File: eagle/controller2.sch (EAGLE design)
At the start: 27 parts, among them K1 SRD-05VDC-SL-C, K2 SRD-05VDC-SL-C, K3 SRD-05VDC-SL-C, K4 SRD-05VDC-SL-C, T1 BC547, T2 BC547, T3 BC547, T4 BC547, X1 VCC, X2 IN1, X3 IN2, X4 IN3, X5 IN4

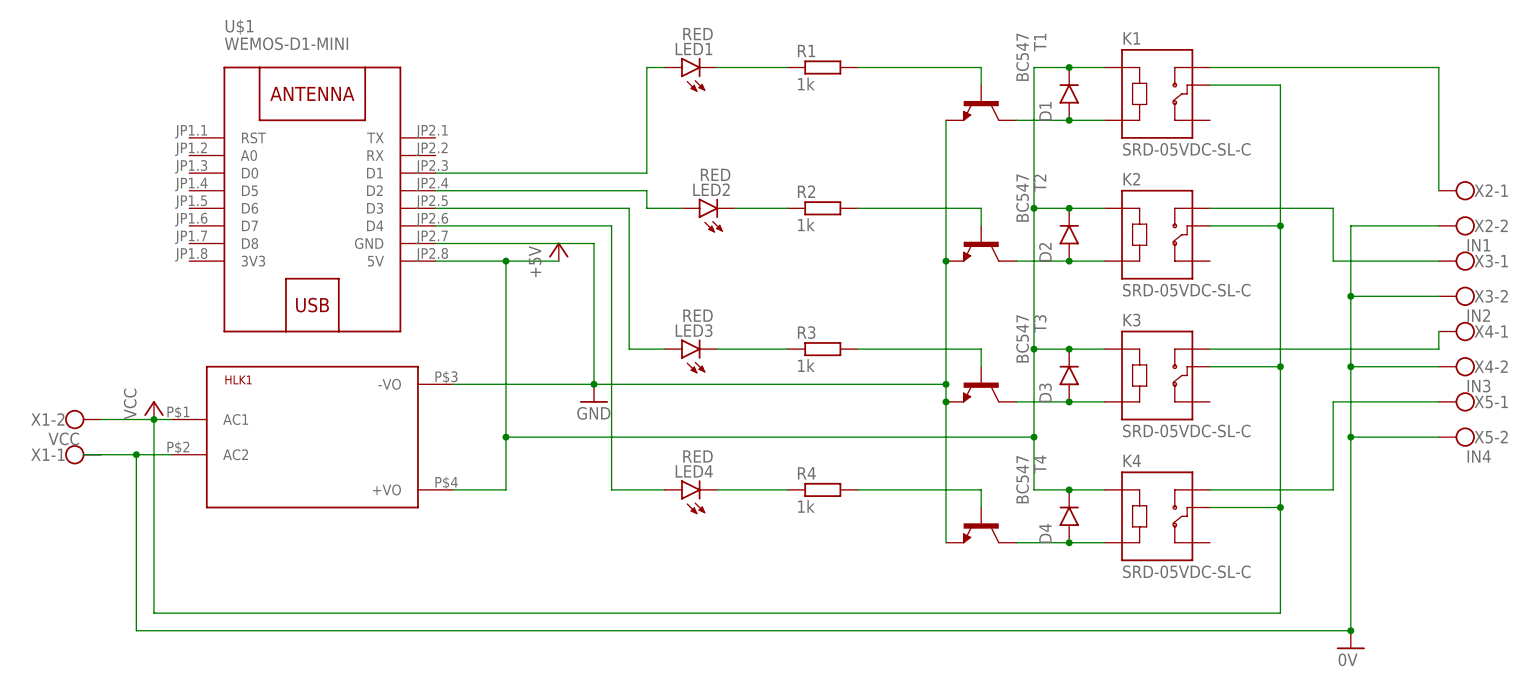
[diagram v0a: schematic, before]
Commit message: Add different board version
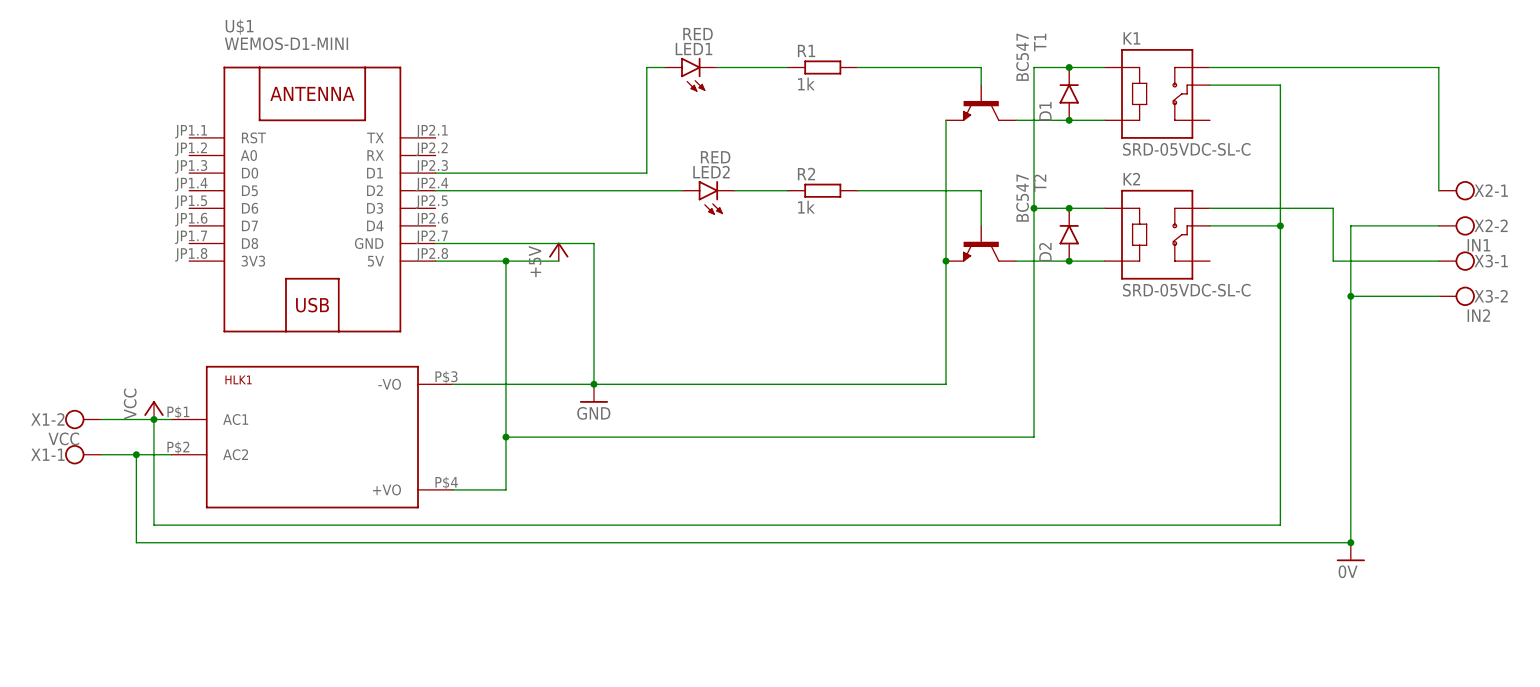
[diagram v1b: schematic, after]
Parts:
- removed D3, D4: 1N4001, tango:1N4001
- removed K3, K4: SRD-05VDC-SL-C, SRD-05VDC-SL-C (1):SRD-05VDC-SL-C
- removed LED3, LED4: RED, led:LED3MM
- removed R3, R4: 1k, rcl:R-EU_0204/5
- removed T3, T4: BC547, transistor:BC547
- removed X4: IN3, con-wago-500:W237-102
- removed X5: IN4, con-wago-500:W237-102
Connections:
- removed net N$10: R4.2, T4.B
- removed net N$12: K3.NO, X4-1.KL
- removed net N$13: K4.NO, X5-1.KL
- removed net N$16: LED3.A, U$1.D3
- removed net N$17: LED4.A, U$1.D4
- removed net N$18: LED3.C, R3.1
- removed net N$4: D3.ANODE, K3.A2, T3.C
- removed net N$5: D4.ANODE, K4.A2, T4.C
- removed net N$6: LED4.C, R4.1
- removed net N$7: R3.2, T3.B
- net +5V: no longer D3.CATHODE, D4.CATHODE, K3.A1, K4.A1
- net 0V: no longer X4-2.KL, X5-2.KL
- net GND: no longer T3.E, T4.E
- net VCC: no longer K3.COM, K4.COM
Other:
- moved on the sheet: LED2, R2
